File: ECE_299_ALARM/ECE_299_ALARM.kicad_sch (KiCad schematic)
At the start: 16 parts, among them SW1 SW_Push_Dual, SW2 SW_Push_Dual, SW3 SW_Push_Dual, SW4 SW_Push_Dual, U1 RDA5807M_Module, U2 RPi_Pico_TH, U3 LM386

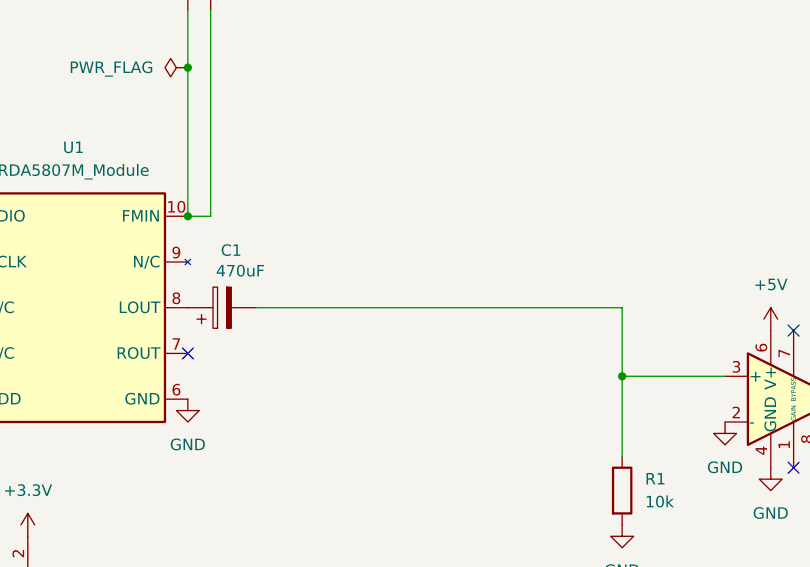
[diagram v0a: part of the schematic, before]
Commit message: i just wasted an hour making better routing
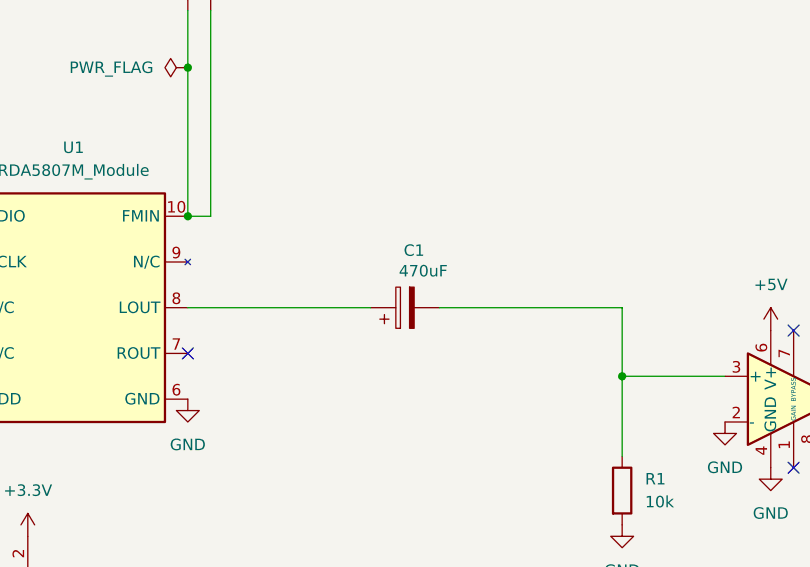
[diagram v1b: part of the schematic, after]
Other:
- moved on the sheet: C1
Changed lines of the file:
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@@
 	(wire
 		(pts
-			(xy 171.45 80.01) (xy 212.09 80.01)
+			(xy 191.77 80.01) (xy 212.09 80.01)
 		)
 		(stroke
@@
 		(pts
 			(xy 109.22 113.03) (xy 130.81 113.03)
+		)
+		(stroke
+			(width 0)
+			(type default)
+		)
+	)
+	(wire
+		(pts
+			(xy 184.15 80.01) (xy 163.83 80.01)
 		)
 		(stroke
@@
 	(symbol
 		(lib_id "Device:C_Polarized")
-		(at 167.64 80.01 90)
+		(at 187.96 80.01 90)
 		(unit 1)
 		(exclude_from_sim no)
@@
 		(dnp no)
 		(property "Reference" "C1"
-			(at 168.656 73.66 90)
+			(at 188.976 73.66 90)
 			(effects
 				(font
@@
 		)
 		(property "Value" "470uF"
-			(at 169.672 75.946 90)
+			(at 189.992 75.946 90)
 			(effects
 				(font
@@
 		)
 		(property "Footprint" "Capacitor_THT:C_Radial_D6.3mm_H11.0mm_P2.50mm"
-			(at 171.45 79.0448 0)
+			(at 191.77 79.0448 0)
 			(effects
 				(font
@@
 		)
 		(property "Datasheet" "~"
-			(at 167.64 80.01 0)
+			(at 187.96 80.01 0)
 			(effects
 				(font
@@
 		)
 		(property "Description" "Polarized capacitor"
-			(at 167.64 80.01 0)
-			(effects
-				(font
+			(at 187.96 80.01 0)
+			(effects
+				(font
